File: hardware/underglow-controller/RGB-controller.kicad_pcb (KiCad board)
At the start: 4 copper layers, 86 x 74.9 mm, 167 parts, among them J2 U.FL-R-SMT-1(10), J3 U.FL-R-SMT-1(10), J4 CONSOLE, J5 U.FL-R-SMT-1(10), J6 DTM1312PA12PBR008, J7 Conn_01x04, J8 Conn_01x05, Q2 STS8DNF3LL, Q3 STS8DNF3LL, Q4 MBT3904DW1T1G, Q5 MBT3904DW1T1G, Q6 Q_PMOS_GDS, SW2 USB BOOT, SW3 SW_Push, SW4 SW_Push, SW5 SW_Push, U2 W25Q128JVS, U3 RP2040, U4 SX1231HIMLTRT, U5 ESP32-S3R2, U6 W25Q128JVS, U7 DRV8844PWP, U8 BD33C0AWFP-CE2, U9 SN65HVD230, Y2 12MHZ, Y3 32mhz, Y4 40MHZ

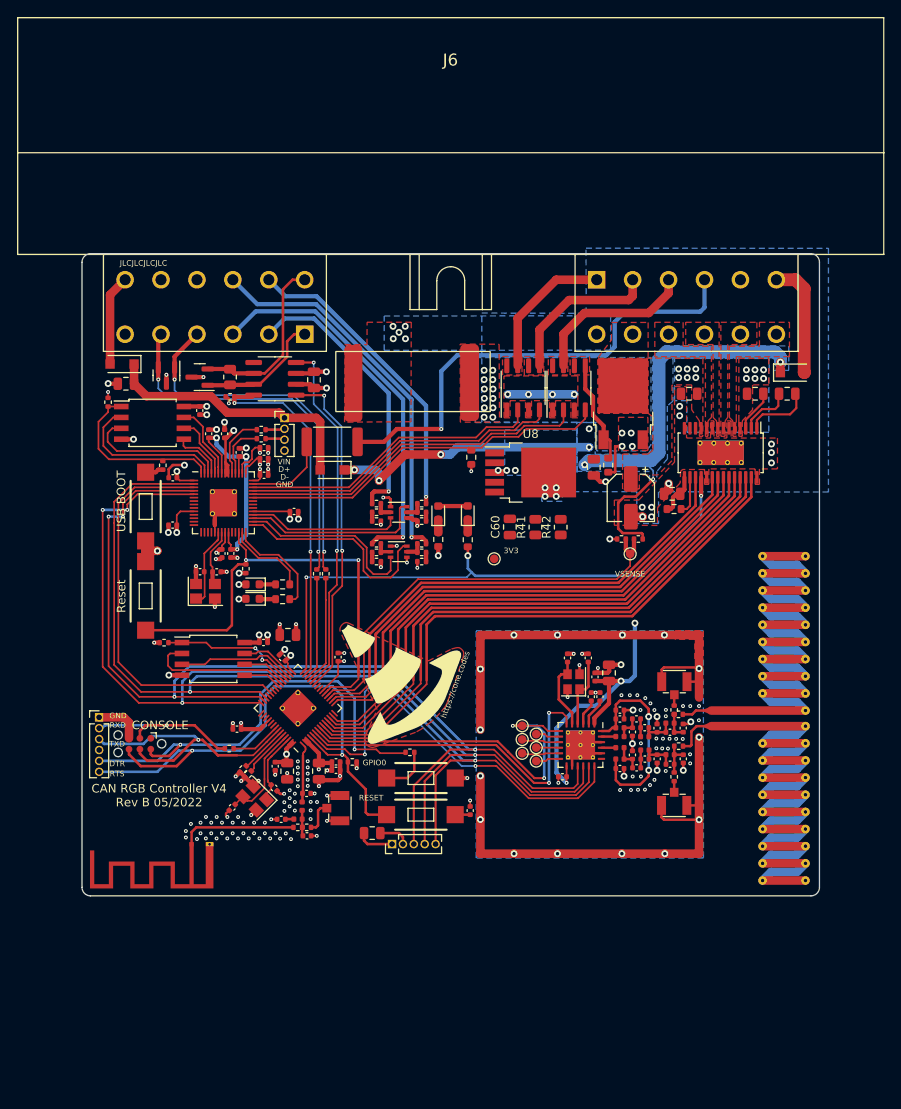
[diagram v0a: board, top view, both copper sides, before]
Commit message: iasdf
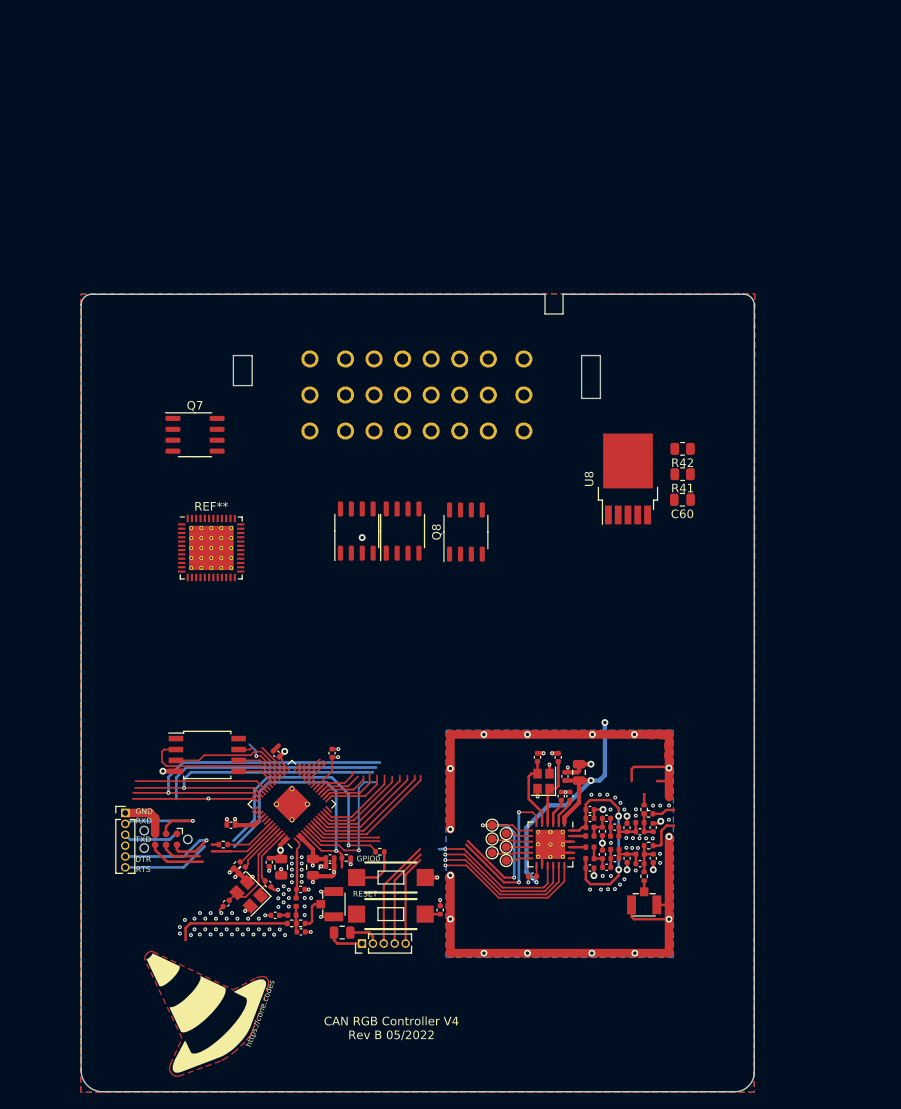
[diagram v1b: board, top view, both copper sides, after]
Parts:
- removed AE2, AE3: Antenna_Shield, RF_Antenna:Texas_SWRA416_868MHz_915MHz
- removed AE4: PCB_ANT, RF_Antenna:Texas_SWRA117D_2.4GHz_Right
- removed C10, C13, C2, C3, C4, C5, C50, C6, C7, C8, C9: 0.1uF, Capacitor_SMD:C_0402_1005Metric
- removed C11, C12: 1uF, Capacitor_SMD:C_0402_1005Metric
- removed C14, C15: 20pF, Capacitor_SMD:C_0402_1005Metric
- removed C42, C56, C61, C62: 10uF, Capacitor_SMD:C_0805_2012Metric
- removed C54: 0.01uF, Capacitor_SMD:C_0805_2012Metric
- removed C55: 0.1uF, Capacitor_SMD:C_0805_2012Metric
- removed C57: 10uF, Capacitor_SMD:CP_Elec_5x5.3
- removed C58: 0.47uF, Capacitor_SMD:C_0805_2012Metric
- removed C59: 1uF, Capacitor_SMD:C_0805_2012Metric
- removed D10, D9: PESD2CANFD24V-T, Package_TO_SOT_SMD:SOT-23
- removed D2, D4, D5: GRN, LED_SMD:LED_0603_1608Metric
- removed D3: RED, LED_SMD:LED_0603_1608Metric
- removed D6, D7, D8: D_Small, Diode_SMD:D_SOD-123F
- removed F2: Fuse, ConeCodes:Keystone-3587-10TR
- removed J2: U.FL-R-SMT-1(10), ConeCodes:HRS_U.FL-R-SMT-1(10)
- removed J7: Conn_01x04, Connector_PinHeader_1.27mm:PinHeader_1x04_P1.27mm_Vertical
- removed Q4, Q5: MBT3904DW1T1G, Package_TO_SOT_SMD:SOT-363_SC-70-6
- removed Q6: Q_PMOS_GDS, Package_TO_SOT_SMD:TO-252-2
- removed R15, R16: 0R, Resistor_SMD:R_0402_1005Metric
- removed R18, R4: 100k, Resistor_SMD:R_0402_1005Metric
- removed R2, R3: 27r4, Resistor_SMD:R_0402_1005Metric
- removed R23, R38, R44: 10k, Resistor_SMD:R_0603_1608Metric
- removed R24: 0R, Resistor_SMD:R_2512_6332Metric
- removed R25, R26, R31, R32, R40, R8: 10k, Resistor_SMD:R_0402_1005Metric
- removed R27, R28, R33, R34, R46, R5: 1k, Resistor_SMD:R_0402_1005Metric
- removed R29, R30, R35, R36: 499R, Resistor_SMD:R_0402_1005Metric
- removed R37, R43, R6, R7: 240R, Resistor_SMD:R_0603_1608Metric
- removed R39: 36k, Resistor_SMD:R_0402_1005Metric
- removed R45: 120,DNF, Resistor_SMD:R_0805_2012Metric
- removed SW2: USB BOOT, ConeCodes:SW_RS-032G05A3-SMRT
- removed SW3: SW_Push, ConeCodes:SW_RS-032G05A3-SMRT
- removed TP8: VSENSE, TestPoint:TestPoint_Pad_D1.0mm
- removed TP9: 3V3OUT, TestPoint:TestPoint_Pad_D1.0mm
- removed U2: W25Q128JVS, Package_SO:SOIC-8W_5.3x5.3mm_P1.27mm
- removed U3: RP2040, ConeCodes:QFN-56
- removed U7: DRV8844PWP, Package_SO:HTSSOP-28-1EP_4.4x9.7mm_P0.65mm_EP2.85x5.4mm_ThermalVias
- removed U9: SN65HVD230, Package_SO:SOIC-8_3.9x4.9mm_P1.27mm
- removed Y2: 12MHZ, Crystal:Crystal_SMD_3225-4Pin_3.2x2.5mm
- added Q7: STS8DNF3LL, Package_SO:SO-8_3.9x4.9mm_P1.27mm, F.Cu at (37.2, 63.1)
- added Q8: STS8DNF3LL, Package_SO:SO-8_3.9x4.9mm_P1.27mm, F.Cu at (68.8, 74.5)
- added REF**: VQFN-48-1EP_7x7mm_P0.5mm_EP5.15x5.15mm_ThermalVias, Package_DFN_QFN:VQFN-48-1EP_7x7mm_P0.5mm_EP5.15x5.15mm_ThermalVias, F.Cu at (39.1, 76.3)
- J6: value DTM1312PA12PBR008 -> Delphi_Sicma_24; footprint ConeCodes:TE_DTM1312PA12PBR008 -> ConeCodes:Delphi_Sicma_24_Black
- moved G*** 44.6 mm to (37.0, 129.1)
- moved Q3 25.6 mm to (61.4, 74.3)
- moved Q2 25.6 mm to (56.0, 74.3)
- moved C60 20.4 mm to (94.0, 70.7), turned to 180 degrees
- moved R41 18.2 mm to (94.0, 67.7), turned to 180 degrees
- moved R42 16.9 mm to (94.0, 64.8), turned to 180 degrees
- moved C21 12.1 mm to (90.6, 108.9)
- moved C22 12.1 mm to (84.7, 109.4)
- moved C27 12.1 mm to (79.9, 105.3)
- moved C28 12.1 mm to (80.9, 105.3)
- moved C30 12.1 mm to (86.1, 112.5)
- moved C32 12.1 mm to (85.2, 113.6)
- moved C33 12.1 mm to (87.6, 112.5)
- moved C34 12.1 mm to (90.6, 112.5)
- moved C35 12.1 mm to (84.7, 112.1)
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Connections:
- net /External-IO/VOUT_EN renamed /External-IO/GPIO4
- J6 pad A1: /Connectors/GPO1 -> unconnected-(J6-PadA1)
- J6 pad A2: /Connectors/GPO2 -> unconnected-(J6-PadA2)
- J6 pad A3: /Connectors/GPO3 -> unconnected-(J6-PadA3)
- J6 pad A4: /Connectors/LEDA -> unconnected-(J6-PadA4)
- J6 pad A5: GND -> unconnected-(J6-PadA5)
- J6 pad A6: /Connectors/IGNITION -> unconnected-(J6-PadA6)
- J6 pad A7: /Connectors/MOTOR1_OUT1 -> unconnected-(J6-PadA7)
- J6 pad A8: /Connectors/MOTOR1_OUT2 -> unconnected-(J6-PadA8)
- J6 pad B1: /CAN_P -> unconnected-(J6-PadB1)
- J6 pad B2: /Connectors/GPI2 -> unconnected-(J6-PadB2)
- J6 pad B3: /Connectors/GPI4 -> unconnected-(J6-PadB3)
- J6 pad B4: /Connectors/USB_D_P -> unconnected-(J6-PadB4)
- J6 pad B5: /Connectors/USB_D_N -> unconnected-(J6-PadB5)
- J6 pad B6: GND -> unconnected-(J6-PadB6)
- J6 pad B7: Net-(D6-Pad2) -> unconnected-(J6-PadB7)
- R10 pad 2: Net-(J2-Pad2) -> unconnected-(R10-Pad2)
- R11 pad 1: Net-(AE3-Pad1) -> unconnected-(R11-Pad1)
- R17 pad 1: Net-(AE4-Pad1) -> unconnected-(R17-Pad1)
- R9 pad 1: Net-(AE2-Pad1) -> unconnected-(R9-Pad1)
- U5 pad 10: /MCPWM0_INB -> /ESP32-S3/GPIO5
- U5 pad 11: /MCPWM0_ENB -> /ESP32-S3/GPIO6
- U5 pad 12: /MCPWM1_INA -> /ESP32-S3/GPIO7
- U5 pad 13: /MCPWM1_ENA -> /ESP32-S3/GPIO8
- U5 pad 15: /MCPWM1_INB -> /ESP32-S3/GPIO10
- U5 pad 16: /MCPWM1_ENB -> /ESP32-S3/GPIO11
- U5 pad 17: /MCPWM_SLEEP -> /ESP32-S3/GPIO12
- U5 pad 28: /MCPWM_FAULT -> /ESP32-S3/SPICS1
- U5 pad 8: /MCPWM0_INA -> /ESP32-S3/GPIO3
- U5 pad 9: /MCPWM0_ENA -> /ESP32-S3/GPIO4
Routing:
- net /VIN: track 82.5 -> 0.00 mm, vias 8 -> 0
- net /MCPWM0_INA: track 69.2 -> 0.00 mm
- net /MCPWM_FAULT: track 68.3 -> 0.00 mm, vias 3 -> 0
- net /MCPWM0_ENA: track 67.8 -> 0.00 mm
- net /MCPWM0_INB: track 66.7 -> 0.00 mm
- net /MCPWM0_ENB: track 65.5 -> 0.00 mm
- net /MCPWM1_INA: track 64.2 -> 0.00 mm
- net /MCPWM1_ENA: track 63.2 -> 0.00 mm
- net /MCPWM1_ENB: track 60.8 -> 0.00 mm
- net /MCPWM1_INB: track 60.6 -> 0.00 mm
- net /MCPWM_SLEEP: track 58.7 -> 0.00 mm
- net GND: track 225.8 -> 167.9 mm, vias 192 -> 138
- net /Connectors/LEDA: track 55.8 -> 0.00 mm, vias 1 -> 0
- net /MISO: track 122.8 -> 69.0 mm, vias 4 -> 2
- net /MOSI: track 118.0 -> 66.1 mm
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- removed copper zone on B.Cu, net /Connectors/FUSE_IN
- removed copper zone on F.Cu, net /Connectors/FUSE_IN
- removed copper zone on B.Cu, net /Connectors/FUSE_OUT
- removed copper zone on F.Cu, net /Connectors/FUSE_OUT
- removed copper zone on F.Cu, net /Connectors/GPO1
- removed copper zone on F.Cu, net /Connectors/GPO2
- removed copper zone on F.Cu, net /Connectors/GPO3
- removed copper zone on F.Cu, net /Connectors/MOTOR1_OUT1
- removed copper zone on F.Cu, net /Connectors/MOTOR1_OUT2
- removed copper zone on F.Cu, net /Connectors/MOTOR2_OUT1
- removed copper zone on F.Cu, net /Connectors/MOTOR2_OUT2
- removed copper zone on B.Cu, net /Connectors/VOUT
- removed copper zone on F.Cu, net /Connectors/VOUT
- removed copper zone on In2.Cu, net /Connectors/VOUT
- removed copper zone on F.Cu, net /External-IO/GPIO4
- removed copper zone on B.Cu, net /VIN
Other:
- board size 86 x 74.9 mm -> 78.5 x 93 mm
- board text removed: "3V3"
- board text removed: "BLUE"
- board text removed: "CAN H"
- board text removed: "CAN L"
- board text removed: "CONSOLE"
- board text removed: "D+"
- board text removed: "D-"
- board text removed: "GPI1"
- board text removed: "GPI2"
- board text removed: "GPI3"
- board text removed: "GPI4"
- board text removed: "GREEN"
- board text removed: "IGN"
- board text removed: "JLCJLCJLCJLC"
- board text removed: "MOTOR1 A"
- board text removed: "MOTOR1 B"
- board text removed: "MOTOR2 A"
- board text removed: "MOTOR2 B"
- board text removed: "RED"
- board text removed: "Reset"
- board text removed: "USB BOOT"
- board text removed: "USB D+"
- board text removed: "USB D-"
- board text removed: "VBATT"
- board text removed: "VIN"
- board text removed: "VOUT"
- board text removed: "VSENSE"
